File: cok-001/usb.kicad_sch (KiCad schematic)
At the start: 37 parts, among them J3301 USB_A_Stacked, J3302 USB_A_Stacked, U3302 BU9869W

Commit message: seperate out
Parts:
- U3303, U3304: footprint Package_SO:SOIC-8_3.9x4.9mm_P1.27mm -> Package_SO:SSOP-8_3.9x5.05mm_P1.27mm
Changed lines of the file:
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@@
 			)
 		)
-		(property "Footprint" "Package_SO:SOIC-8_3.9x4.9mm_P1.27mm"
+		(property "Footprint" "Package_SO:SSOP-8_3.9x5.05mm_P1.27mm"
 			(at 181.61 48.26 0)
 			(effects
@@
 			)
 		)
-		(property "Footprint" "Package_SO:SOIC-8_3.9x4.9mm_P1.27mm"
+		(property "Footprint" "Package_SO:SSOP-8_3.9x5.05mm_P1.27mm"
 			(at 175.26 118.11 0)
 			(effects

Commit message: update to 9
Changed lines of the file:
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@@
 (kicad_sch
-	(version 20231120)
+	(version 20250114)
 	(generator "eeschema")
-	(generator_version "8.0")
+	(generator_version "9.0")
 	(paper "A4")
 	(junction

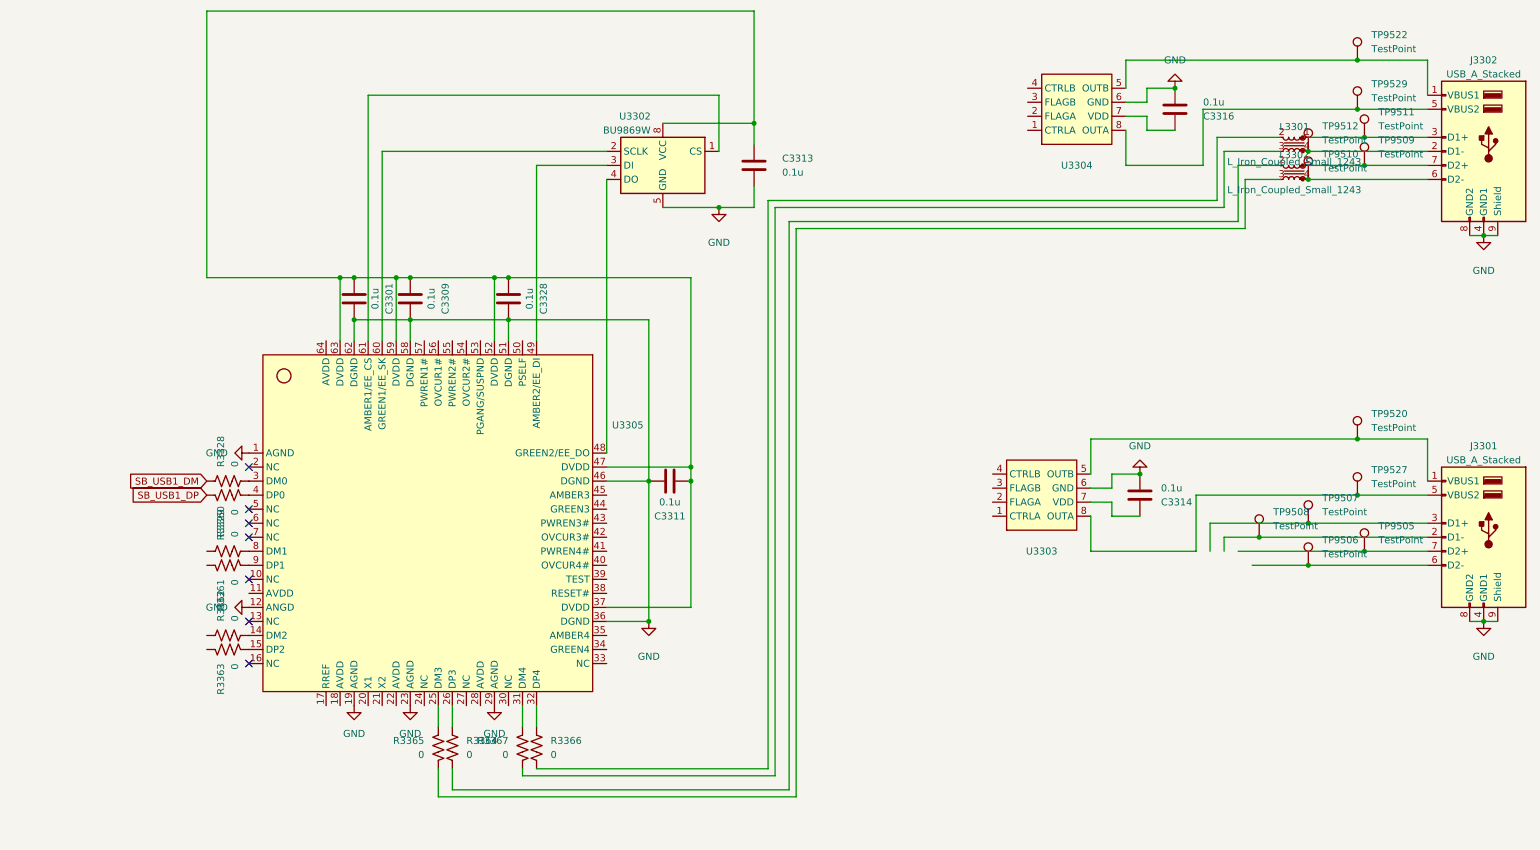
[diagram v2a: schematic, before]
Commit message: led
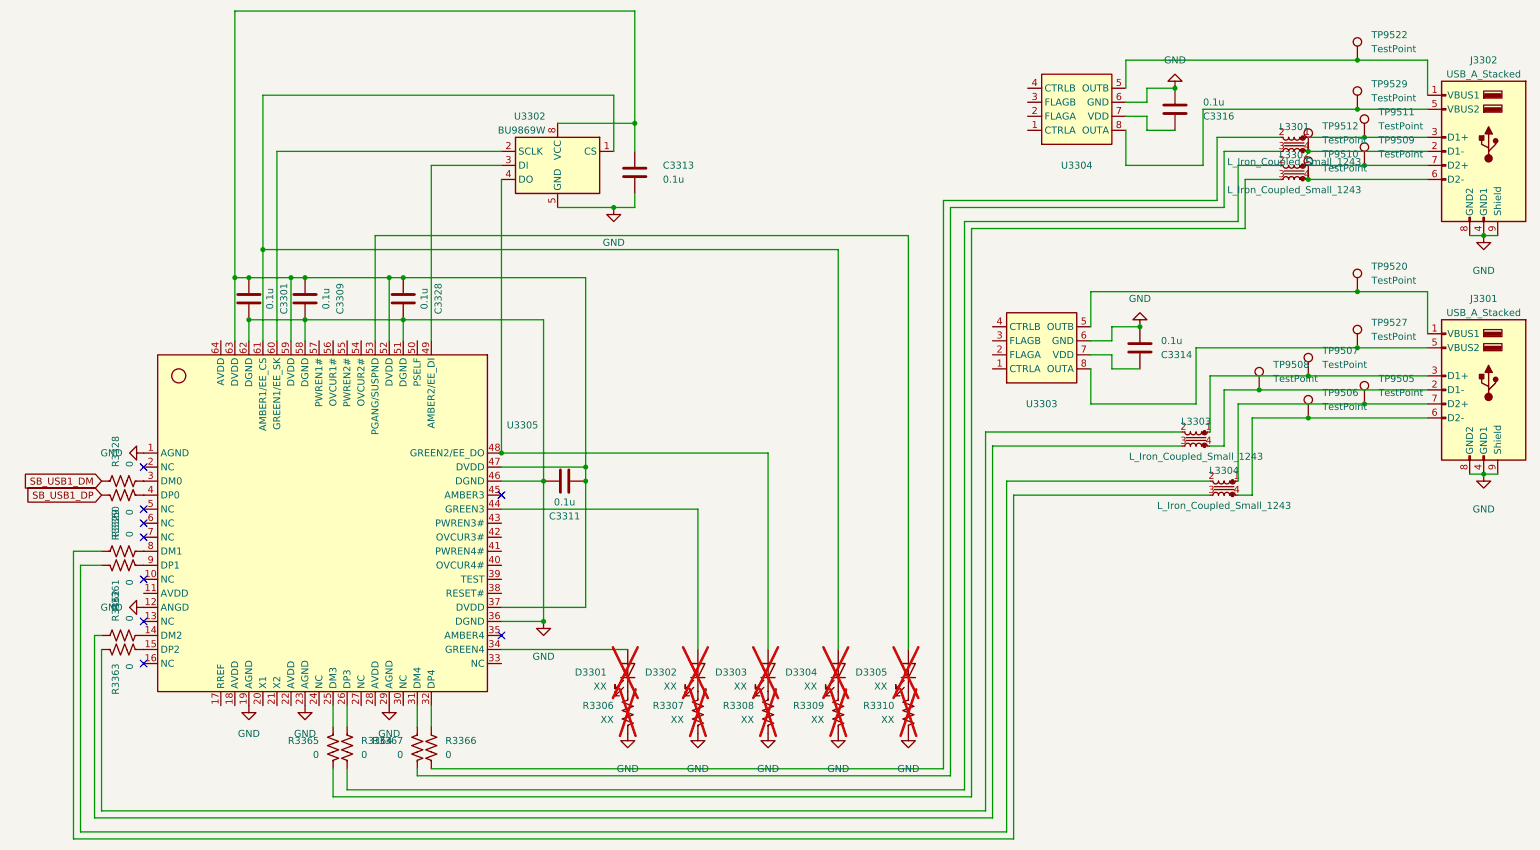
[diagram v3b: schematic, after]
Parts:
- added D3301, D3302, D3303, D3304, D3305: XX, Diode_SMD:D_0603_1608Metric, symbol Device:LED
- added L3303, L3304: L_Iron_Coupled_Small_1243, Inductor_SMD:L_CommonModeChoke_Coilcraft_0805USB, symbol Device:L_Iron_Coupled_Small_1243
- added R3306, R3307, R3308, R3309, R3310: XX, Resistor_SMD:R_0402_1005Metric, symbol Device:R_US
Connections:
- net GND: now also R3306.1, R3307.1, R3308.1, R3309.1, R3310.1
- net at J3301.2 (D1-), TP9508.1: now also L3303.4
- net at J3301.3 (D1+), TP9507.1: now also L3303.1
- net at J3301.6 (D2-), TP9506.1: now also L3304.4
- net at J3301.7 (D2+), TP9505.1: now also L3304.1
- net at R3363.2: now also L3303.2
- net at U3302.1 (CS), U3305.61 (AMBER1/EE_CS): now also D3304.2 (A)
- net at U3302.4 (DO), U3305.48 (GREEN2/EE_DO): now also D3303.2 (A)
- net at U3305.34 (GREEN4): now also D3301.2 (A)
- net at U3305.44 (GREEN3): now also D3302.2 (A)
- net at U3305.53 (PGANG/SUSPND): now also D3305.2 (A)
- net at R3362.2: now also L3303.3
- net at R3360.2: now also L3304.3
- net at R3361.2: now also L3304.2
- new net: D3304.1 (K), R3309.2
- new net: D3303.1 (K), R3308.2
- new net: D3302.1 (K), R3307.2
- new net: D3305.1 (K), R3310.2
- new net: D3301.1 (K), R3306.2
- no-connect marks 7 -> 9
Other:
- moved on the sheet: C3301, C3309, C3311, C3313, C3314, C3328, J3301, R3328, R3329, R3360, R3361, R3362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
